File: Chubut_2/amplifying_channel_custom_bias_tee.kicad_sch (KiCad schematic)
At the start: 6 parts

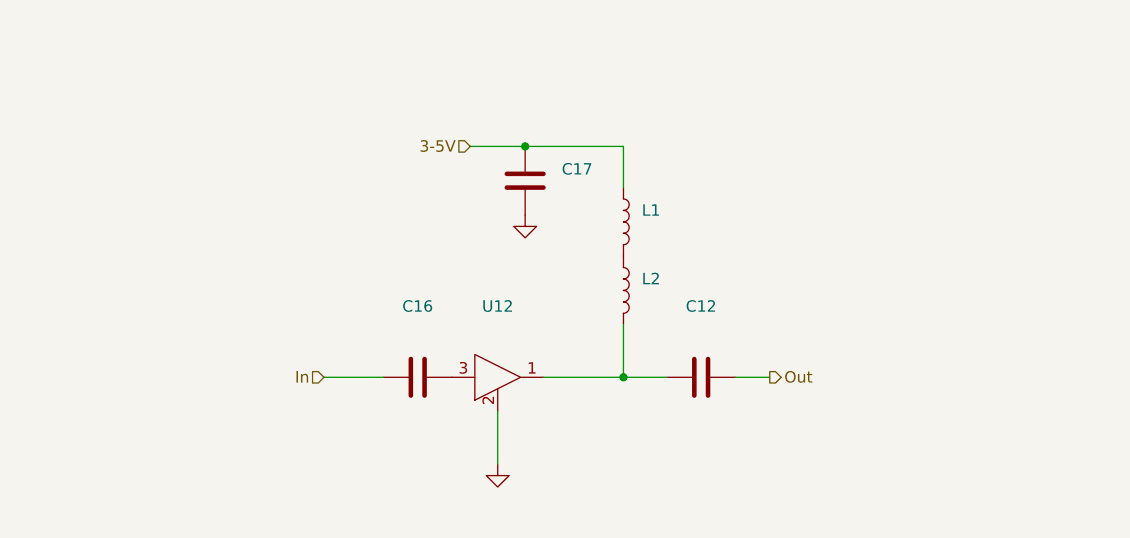
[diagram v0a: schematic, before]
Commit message: Several updates
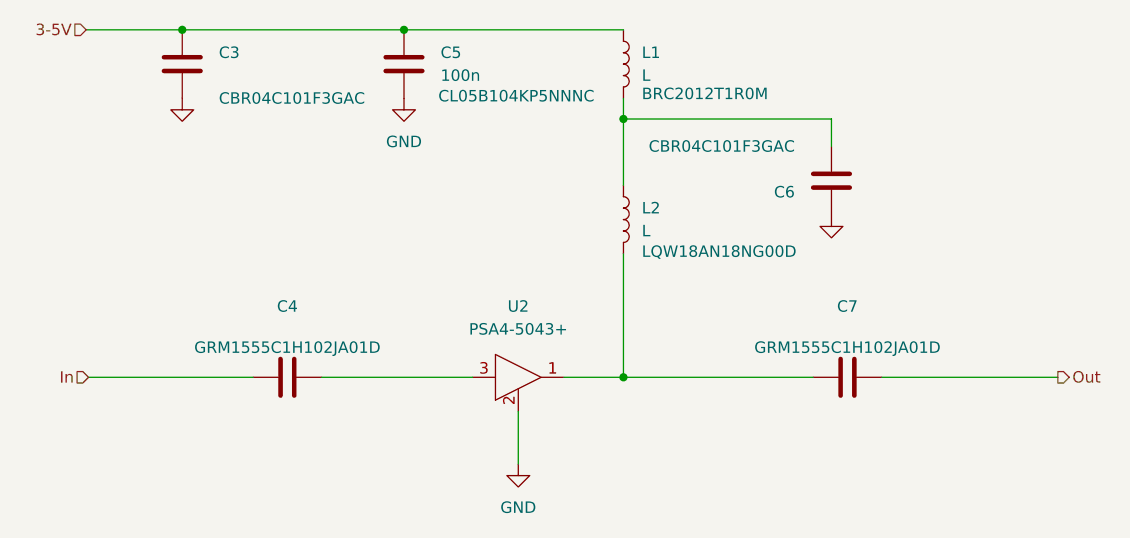
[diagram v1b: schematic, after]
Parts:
- removed C12, C16: (no value), symbol Device:C
- added C3, C4, C6, C7: (no value), symbol Device:C
- C5: renamed from C17; value (none) -> 100n; footprint (none) -> Capacitor_SMD:C_0805_2012Metric; Manufacturer (none) -> Samsung Electro-Mechanics; Manufacturer number (none) -> CL05B104KP5NNNC
- L1: value (none) -> L; footprint (none) -> Inductor_SMD:L_0402_1005Metric; Manufacturer (none) -> Taiyo Yuden; Manufacturer number (none) -> BRC2012T1R0M
- L2: value (none) -> L; footprint (none) -> Inductor_SMD:L_0402_1005Metric; Manufacturer (none) -> Murata Electronics; Manufacturer number (none) -> LQW18AN18NG00D
- U2: renamed from U12; value (none) -> PSA4-5043+; footprint (none) -> chubut:MMM1362; Manufacturer (none) -> Mini-Circuits; Manufacturer number (none) -> PSA4-5043+
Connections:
- net 3-5V: now also C3.1
- net GND: now also C3.2, C6.1
- net In: now also C4.1
- net Out: now also C7.2
- net at U2.3 (RF-IN): now also C4.2
- net at L1.2, L2.1: now also C6.2
- net at L2.2, U2.1 (RF-OUT_and_DC-IN): now also C7.1
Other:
- moved on the sheet: C5, L1, L2, U2
